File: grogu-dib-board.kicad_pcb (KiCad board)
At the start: 4 copper layers, 9.5 x 102.6 mm, 18 parts, among them J1 ERF8-050-05.0-L-DV-K-TR, J2 ERF8-050-05.0-L-DV-K-TR

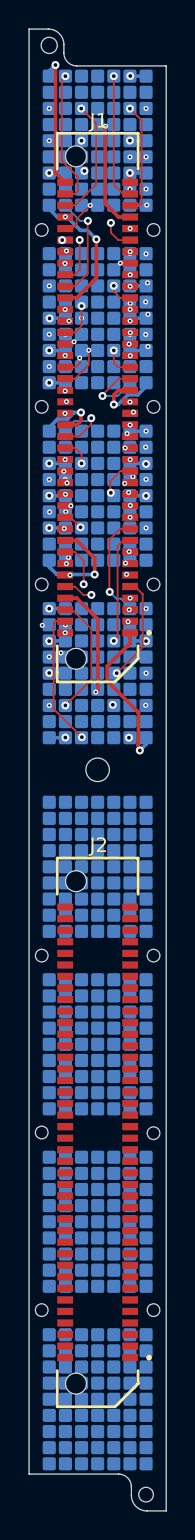
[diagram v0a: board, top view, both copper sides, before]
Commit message: more routing
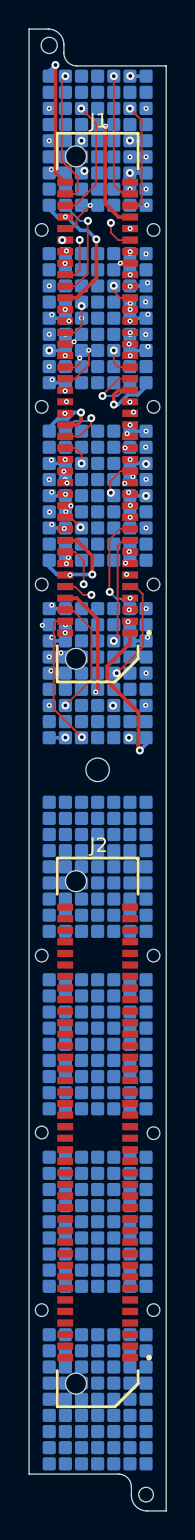
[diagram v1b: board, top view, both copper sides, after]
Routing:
- net /FB3.LF: track 12.3 -> 12.2 mm, vias 18 -> 27
- net /FB2.LF: vias 21 -> 22
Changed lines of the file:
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@@
 	)
 	(via
-		(at 74.5066 86.5564)
+		(at 74.5236 86.614)
 		(size 0.5588)
 		(drill 0.254)
@@
 	)
 	(segment
+		(start 74.868021 79.970597)
+		(end 75.158719 79.970597)
+		(width 0.127)
+		(layer "In2.Cu")
+		(net 20)
+	)
+	(segment
+		(start 74.5236 86.614)
+		(end 74.041 86.1314)
+		(width 0.127)
+		(layer "In2.Cu")
+		(net 20)
+	)
+	(segment
+		(start 74.041 86.1314)
+		(end 74.041 80.797618)
+		(width 0.127)
+		(layer "In2.Cu")
+		(net 20)
+	)
+	(segment
 		(start 74.041 80.797618)
-		(end 74.041 86.0908)
-		(width 0.127)
-		(layer "In2.Cu")
-		(net 20)
-	)
-	(segment
-		(start 74.041 86.0908)
-		(end 74.5066 86.5564)
-		(width 0.127)
-		(layer "In2.Cu")
-		(net 20)
-	)
-	(segment
-		(start 75.158719 79.970597)
 		(end 74.868021 79.970597)
-		(width 0.127)
-		(layer "In2.Cu")
-		(net 20)
-	)
-	(segment
-		(start 74.868021 79.970597)
-		(end 74.041 80.797618)
 		(width 0.127)
 		(layer "In2.Cu")
@@
 	)
 	(via blind
-		(at 70.1294 59.7916)
+		(at 69.964146 69.980048)
+		(size 0.5588)
+		(drill 0.254)
+		(layers "In1.Cu" "In2.Cu")
+		(net 395)
+	)
+	(via blind
+		(at 69.964146 49.863248)
+		(size 0.5588)
+		(drill 0.254)
+		(layers "In1.Cu" "In2.Cu")
+		(net 395)
+	)
+	(via blind
+		(at 69.989546 72.215248)
+		(size 0.5588)
+		(drill 0.254)
+		(layers "In1.Cu" "In2.Cu")
+		(net 395)
+	)
+	(via blind
+		(at 70.1058 62.0141)
 		(size 0.5588)
 		(drill 0.254)
@@
 	)
 	(via blind
-		(at 70.1058 74.3077)
-		(size 0.5588)
-		(drill 0.254)
-		(layers "In1.Cu" "B.Cu")
-		(net 395)
-	)
-	(via blind
-		(at 70.1058 79.8957)
-		(size 0.5588)
-		(drill 0.254)
-		(layers "In1.Cu" "B.Cu")
-		(net 395)
-	)
-	(via blind
-		(at 70.1058 64.2493)
-		(size 0.5588)
-		(drill 0.254)
-		(layers "In1.Cu" "B.Cu")
-		(net 395)
-	)
-	(via blind
-		(at 70.1058 72.0725)
-		(size 0.5588)
-		(drill 0.254)
-		(layers "In1.Cu" "B.Cu")
-		(net 395)
-	)
-	(via blind
-		(at 70.1058 62.0141)
-		(size 0.5588)
-		(drill 0.254)
-		(layers "In1.Cu" "B.Cu")
-		(net 395)
-	)
-	(via blind
-		(at 70.1058 69.8373)
-		(size 0.5588)
-		(drill 0.254)
-		(layers "In1.Cu" "B.Cu")
-		(net 395)
-	)
-	(via blind
-		(at 70.1058 49.7205)
-		(size 0.5588)
-		(drill 0.254)
-		(layers "In1.Cu" "B.Cu")
-		(net 395)
-	)
-	(via blind
-		(at 70.104 84.3534)
-		(size 0.5588)
-		(drill 0.254)
-		(layers "In1.Cu" "B.Cu")
-		(net 395)
-	)
-	(via blind
-		(at 70.104 82.1436)
-		(size 0.5588)
-		(drill 0.254)
-		(layers "In1.Cu" "B.Cu")
+		(at 70.014946 64.417448)
+		(size 0.5588)
+		(drill 0.254)
+		(layers "In1.Cu" "In2.Cu")
+		(net 395)
+	)
+	(via blind
+		(at 69.989546 59.921648)
+		(size 0.5588)
+		(drill 0.254)
+		(layers "In1.Cu" "In2.Cu")
+		(net 395)
+	)
+	(via blind
+		(at 69.989546 74.450448)
+		(size 0.5588)
+		(drill 0.254)
+		(layers "In1.Cu" "In2.Cu")
+		(net 395)
+	)
+	(via blind
+		(at 69.989546 82.273648)
+		(size 0.5588)
+		(drill 0.254)
+		(layers "In1.Cu" "In2.Cu")
+		(net 395)
+	)
+	(via blind
+		(at 69.989546 80.038448)
+		(size 0.5588)
+		(drill 0.254)
+		(layers "In1.Cu" "In2.Cu")
+		(net 395)
+	)
+	(via blind
+		(at 69.937674 84.587033)
+		(size 0.5588)
+		(drill 0.254)
+		(layers "In1.Cu" "In2.Cu")
+		(net 395)
+	)
+	(via micro
+		(at 70.2564 49.4792)
+		(size 0.3556)
+		(drill 0.1524)
+		(layers "In2.Cu" "B.Cu")
+		(net 395)
+	)
+	(via micro
+		(at 70.2818 74.0664)
+		(size 0.3556)
+		(drill 0.1524)
+		(layers "In2.Cu" "B.Cu")
+		(net 395)
+	)
+	(via micro
+		(at 70.2818 59.5376)
+		(size 0.3556)
+		(drill 0.1524)
+		(layers "In2.Cu" "B.Cu")
+		(net 395)
+	)
+	(via micro
+		(at 70.3072 64.0334)
+		(size 0.3556)
+		(drill 0.1524)
+		(layers "In2.Cu" "B.Cu")
+		(net 395)
+	)
+	(via micro
+		(at 70.2564 69.596)
+		(size 0.3556)
+		(drill 0.1524)
+		(layers "In2.Cu" "B.Cu")
+		(net 395)
+	)
+	(via micro
+		(at 70.2818 81.8896)
+		(size 0.3556)
+		(drill 0.1524)
+		(layers "In2.Cu" "B.Cu")
+		(net 395)
+	)
+	(via micro
+		(at 70.229928 84.202985)
+		(size 0.3556)
+		(drill 0.1524)
+		(layers "In2.Cu" "B.Cu")
+		(net 395)
+	)
+	(via micro
+		(at 70.2818 71.8312)
+		(size 0.3556)
+		(drill 0.1524)
+		(layers "In2.Cu" "B.Cu")
+		(net 395)
+	)
+	(via micro
+		(at 70.2818 79.6544)
+		(size 0.3556)
+		(drill 0.1524)
+		(layers "In2.Cu" "B.Cu")
+		(net 395)
+	)
+	(segment
+		(start 70.229928 84.202985)
+		(end 70.393043 84.3661)
+		(width 0.254)
+		(layer "B.Cu")
 		(net 395)
 	)
@@
 	)
 	(segment
-		(start 71.2234 84.3661)
-		(end 70.1058 84.3661)
+		(start 70.393043 84.3661)
+		(end 71.2234 84.3661)
 		(width 0.254)
 		(layer "B.Cu")
@@
 	)
 	(segment
-		(start 73.253503 77.533499)
-		(end 73.253503 76.410328)
-		(width 0.254)
-		(layer "F.Cu")
-		(net 402)
-	)
-	(segment
-		(start 73.253503 76.410328)
+		(start 73.0885 76.245325)
 		(end 72.011875 75.1687)
 		(width 0.254)
@@
 		(net 402)
 	)
-	(via
-		(at 73.253503 77.533499)
-		(size 0.5588)
-		(drill 0.254)
-		(layers "F.Cu" "B.Cu")
+	(segment
+		(start 73.0885 77.532247)
+		(end 73.0885 76.245325)
+		(width 0.254)
+		(layer "F.Cu")
 		(net 402)
 	)
-	(segment
-		(start 73.253503 77.533499)
-		(end 70.6392 77.533499)
+	(via
+		(at 73.0885 77.532247)
+		(size 0.5588)
+		(drill 0.254)
+		(layers "F.Cu" "B.Cu")
+		(net 402)
+	)
+	(segment
+		(start 70.637948 77.532247)
+		(end 70.1058 77.000099)
+		(width 0.254)
+		(layer "B.Cu")
+		(net 402)
+	)
+	(segment
+		(start 73.0885 77.532247)
+		(end 70.637948 77.532247)
 		(width 0.254)
 		(layer "B.Cu")
@@
 	)
 	(segment
-		(start 70.6392 77.533499)
-		(end 70.1058 77.000099)
-		(width 0.254)
-		(layer "B.Cu")
-		(net 402)
-	)
-	(segment
 		(start 72.305217 66.3067)
 		(end 72.305217 66.875358)
@@
 	)
 	(via blind
-		(at 76.8096 82.1436)
+		(at 76.708 57.7596)
+		(size 0.5588)
+		(drill 0.254)
+		(layers "In1.Cu" "In2.Cu")
+		(free yes)
+		(net 405)
+	)
+	(via blind
+		(at 76.7334 62.1792)
+		(size 0.5588)
+		(drill 0.254)
+		(layers "In1.Cu" "In2.Cu")
+		(free yes)
+		(net 405)
+	)
+	(via blind
+		(at 76.8096 69.8754)
 		(size 0.5588)
 		(drill 0.254)
@@
 	)
 	(via blind
-		(at 76.708 57.7596)
+		(at 76.706068 82.376299)
 		(size 0.5588)
 		(drill 0.254)
@@
 	)
 	(via blind
-		(at 76.7334 62.1792)
+		(at 76.835 59.9948)
 		(size 0.5588)
 		(drill 0.254)
@@
 		(net 405)
 	)
-	(via blind
-		(at 76.8096 69.8754)
-		(size 0.5588)
-		(drill 0.254)
-		(layers "In1.Cu" "B.Cu")
+	(via micro
+		(at 76.941857 61.743941)
+		(size 0.3556)
+		(drill 0.1524)
+		(layers "In2.Cu" "B.Cu")
 		(net 405)
 	)
-	(via blind
-		(at 76.835 59.9948)
-		(size 0.5588)
-		(drill 0.254)
-		(layers "In1.Cu" "In2.Cu")
-		(free yes)
+	(via micro
+		(at 76.8114 67.6021)
+		(size 0.3556)
+		(drill 0.1524)
+		(layers "In2.Cu" "B.Cu")
 		(net 405)
 	)
 	(via micro
-		(at 76.941857 61.743941)
-		(size 0.3556)
-		(drill 0.1524)
-		(layers "In2.Cu" "B.Cu")
-		(net 405)
-	)
-	(via micro
-		(at 76.8114 67.6021)
-		(size 0.3556)
-		(drill 0.1524)
+		(at 76.916457 81.886141)
+		(size 0.3556)
+		(drill 0.1524)
